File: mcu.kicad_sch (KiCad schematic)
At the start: 35 parts, among them J6 DEBUG, Q1 BSS138DW, Q2 BSS138DW, SW2 El Button, U3 GW J9LHS2.4M-C0C7-2+35+13+40A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, U4 BMD-340, U5 XT25F128F

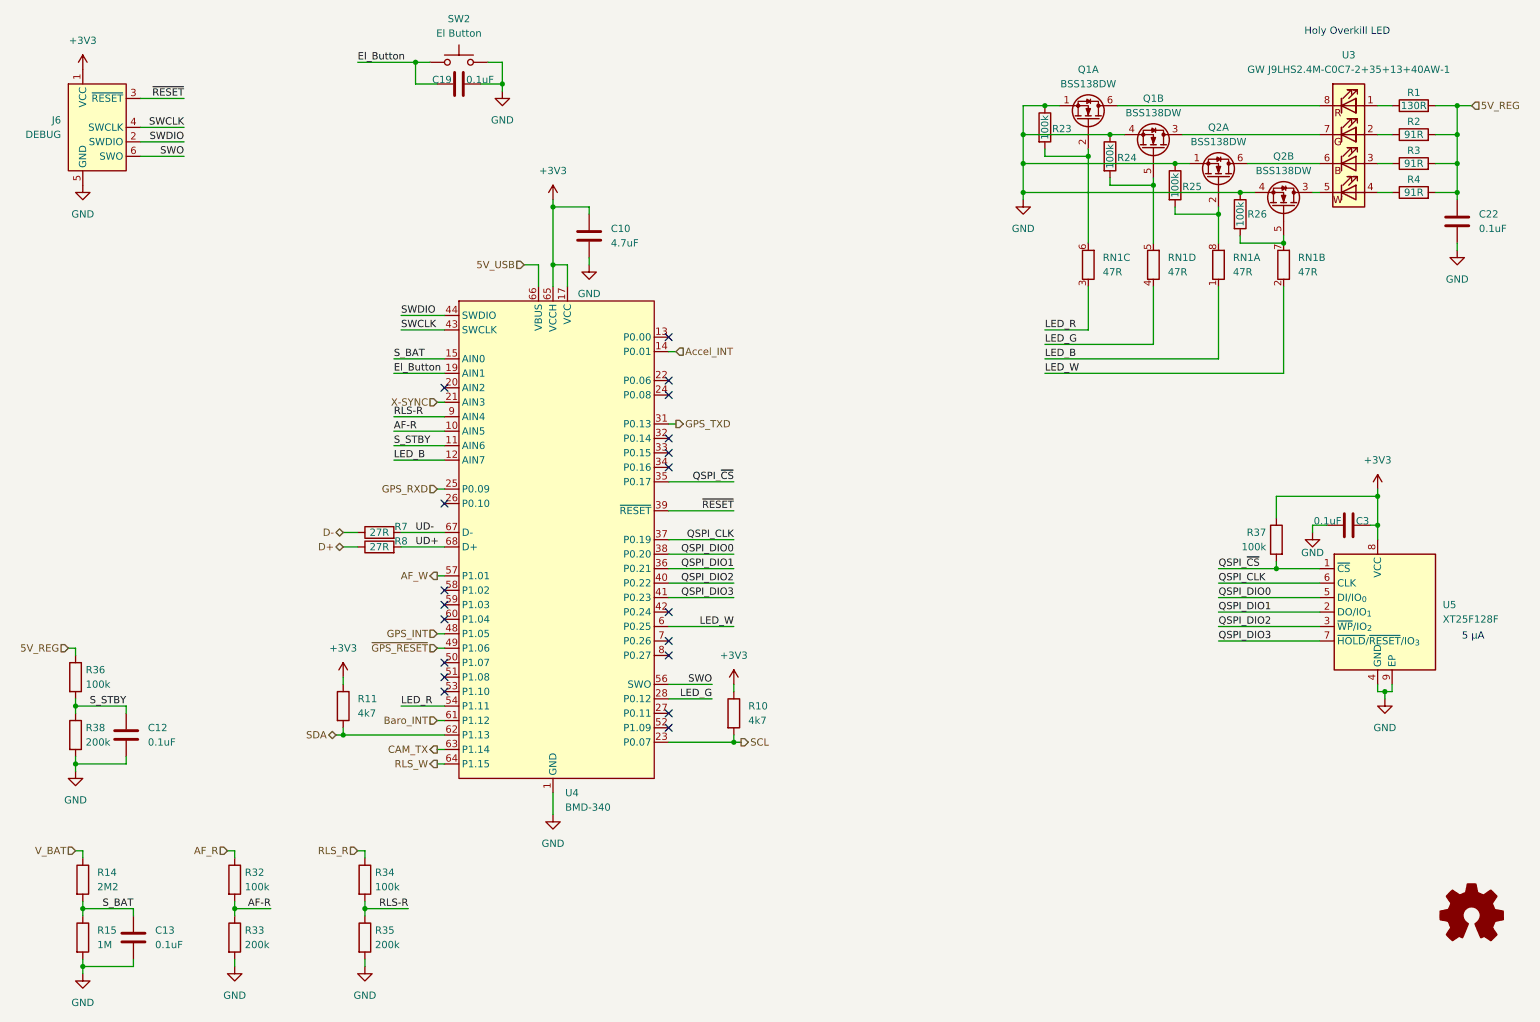
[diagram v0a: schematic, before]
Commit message: idk
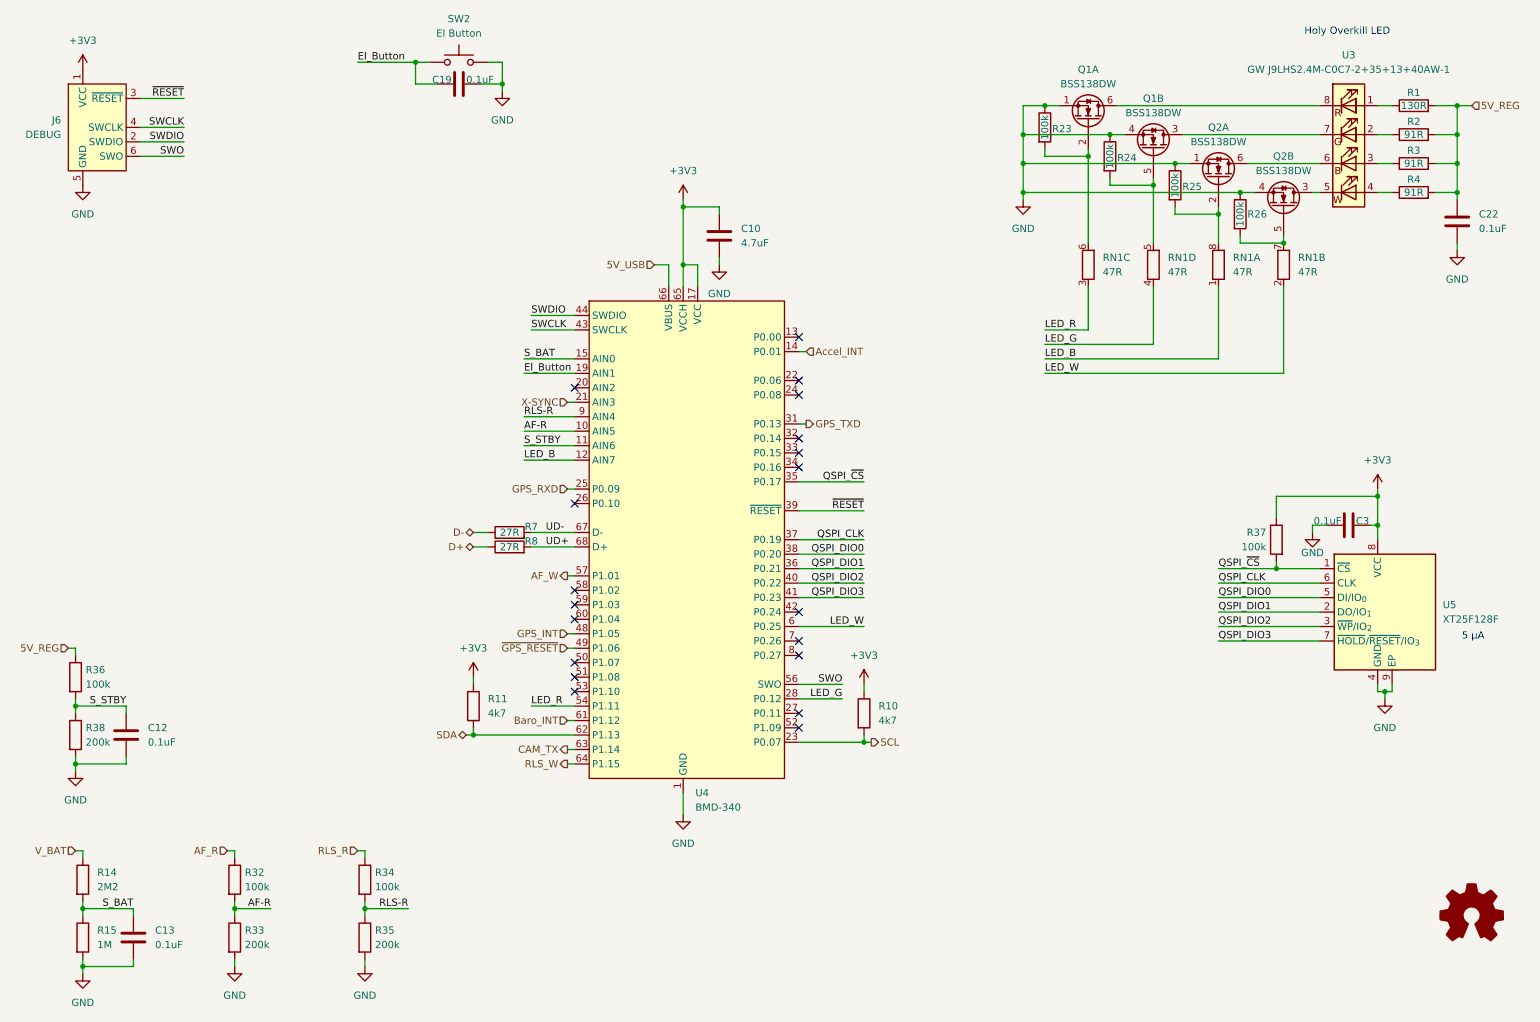
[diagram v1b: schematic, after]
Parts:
- R7, R8: LCSC C25100 -> C2909343
- U4: LCSC (none) -> C5456944
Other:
- moved on the sheet: C10, R10, R11, R7, R8, U4
